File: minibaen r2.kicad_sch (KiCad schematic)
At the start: 134 parts, among them SW1 SW_Push, SW2 RotaryEncoder_Switch, U1 ATmega32U2-A, U2 PRTR5V0U2X, Y1 Crystal_GND24_Small

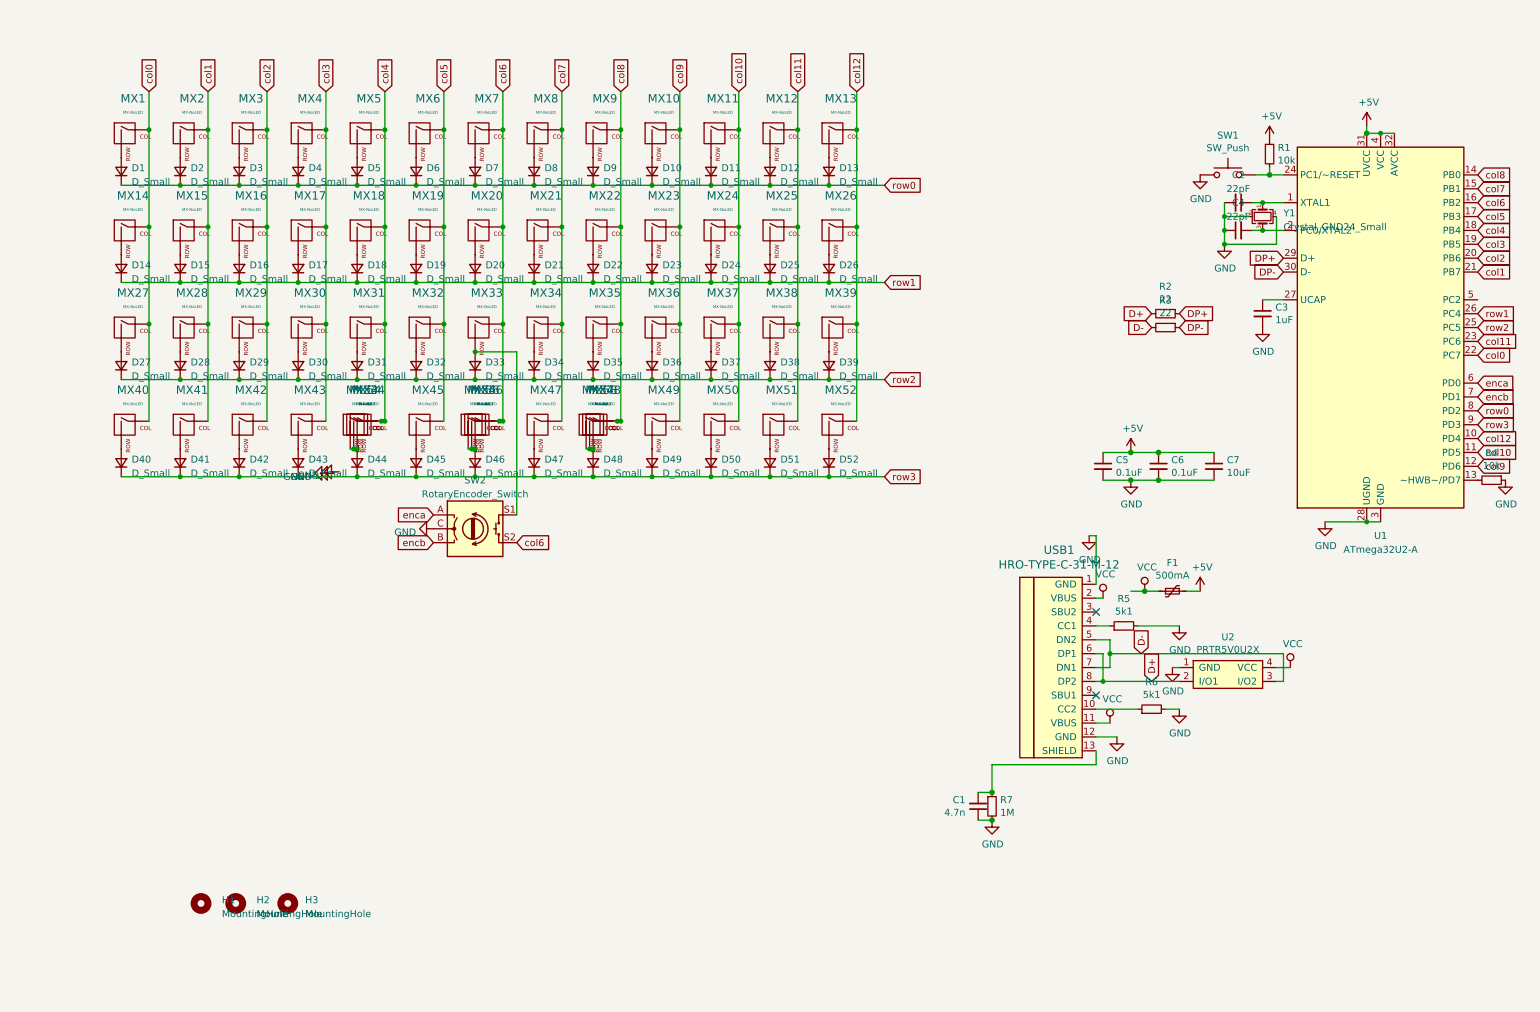
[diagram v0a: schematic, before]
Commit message: stagger
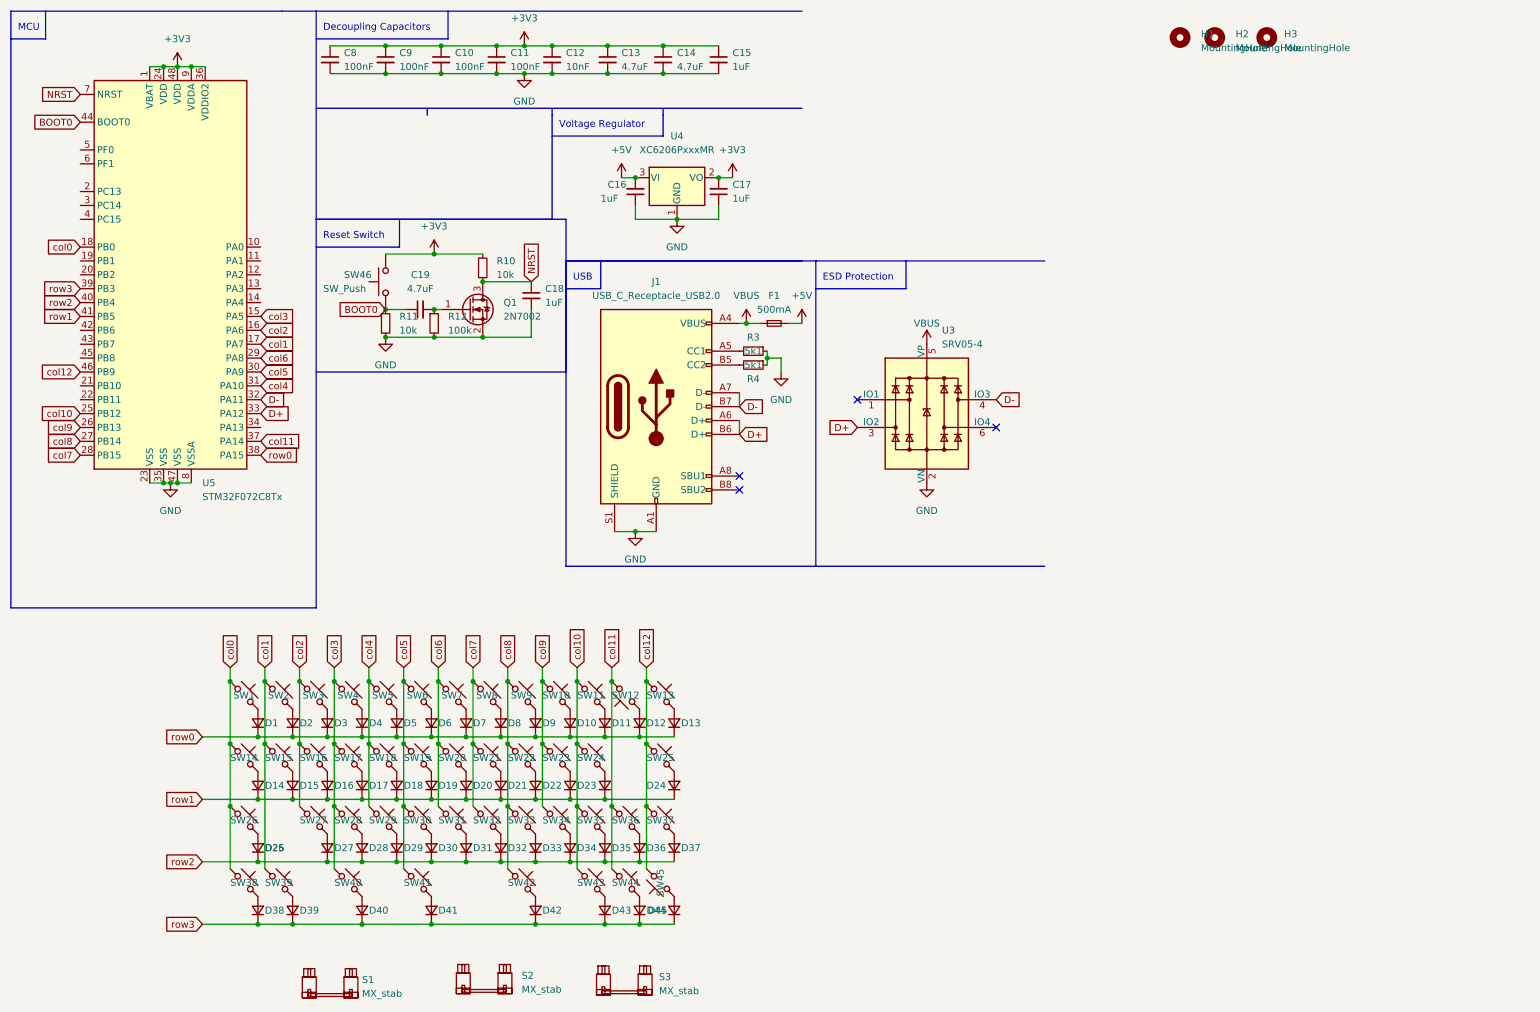
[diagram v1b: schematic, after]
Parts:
- removed C1: 4.7n, Capacitor_SMD:C_0603_1608Metric, symbol Device:C_Small
- removed C2, C4: 22pF, Capacitor_SMD:C_0603_1608Metric, symbol Device:C_Small
- removed C3: 1uF, Capacitor_SMD:C_0603_1608Metric, symbol Device:C_Small
- removed C5, C6: 0.1uF, Capacitor_SMD:C_0603_1608Metric, symbol Device:C_Small
- removed C7: 10uF, Capacitor_SMD:C_0603_1608Metric, symbol Device:C_Small
- removed D46, D47, D48, D49, D50, D51, D52: D_Small, Diode_SMD:D_SOD-123, symbol Device:D_Small
- removed F1: 500mA, Fuse:Fuse_1206_3216Metric, symbol Device:Polyfuse_Small
- removed MX1, MX10, MX11, MX12, MX13, MX14, MX15, MX16, MX17, MX18, MX19, MX2, MX20, MX21, MX22, MX23, MX24, MX25, MX26, MX27, MX28, MX29, MX3, MX30, MX31, MX32, MX33, MX34, MX35, MX36, MX37, MX38, MX39, MX4, MX40, MX41, MX42, MX43, MX44, MX45, MX46, MX47, MX48, MX49, MX5, MX50, MX51, MX52, MX6, MX7, MX8, MX9: MX-NoLED, MX_Only:MXOnly-1U-NoLED, symbol keybage:MX-NoLED
- removed MX53, MX57: MX-NoLED, MX_Only:MXOnly-2U-ReversedStabilizers-NoLED, symbol keybage:MX-NoLED
- removed MX54, MX56, MX58: MX-NoLED, MX_Only:MXOnly-3U-ReversedStabilizers-NoLED, symbol keybage:MX-NoLED
- removed MX55: MX-NoLED, MX_Only:MXOnly-7U-ReversedStabilizers-NoLED, symbol keybage:MX-NoLED
- removed R1: 10k, Resistor_SMD:R_0603_1608Metric, symbol Device:R_Small
- removed R2: 22, Resistor_SMD:R_0603_1608Metric, symbol Device:R_Small
- removed R5, R6: 5k1, Resistor_SMD:R_0603_1608Metric, symbol Device:R_Small
- removed R7: 1M, Resistor_SMD:R_0603_1608Metric, symbol Device:R_Small
- removed SW1: SW_Push, Connector_PinHeader_2.54mm:PinHeader_1x02_P2.54mm_Vertical, symbol Switch:SW_Push
- removed SW2: RotaryEncoder_Switch, keebio:RotaryEncoder_EC11-no-legs, symbol Device:RotaryEncoder_Switch
- removed U1: ATmega32U2-A, Package_QFP:TQFP-32_7x7mm_P0.8mm, symbol MCU_Microchip_ATmega:ATmega32U2-A
- removed U2: PRTR5V0U2X, Package_TO_SOT_SMD:SOT-143, symbol keebio:PRTR5V0U2X
- removed USB1: HRO-TYPE-C-31-M-12, Type-C:HRO-TYPE-C-31-M-12, symbol Type-C:HRO-TYPE-C-31-M-12
- removed Y1: Crystal_GND24_Small, Crystal:Crystal_SMD_3225-4Pin_3.2x2.5mm, symbol Device:Crystal_GND24_Small
- added C10, C11, C8, C9: 100nF, Capacitor_SMD:C_0402_1005Metric, symbol Device:C_Small
- added C12: 10nF, Capacitor_SMD:C_0402_1005Metric, symbol Device:C_Small
- added C13, C14, C19: 4.7uF, Capacitor_SMD:C_0402_1005Metric, symbol Device:C_Small
- added C15, C16, C17, C18: 1uF, Capacitor_SMD:C_0402_1005Metric, symbol Device:C_Small
- added F1: 500mA, Fuse:Fuse_0603_1608Metric, symbol Device:Fuse_Small
- added J1: USB_C_Receptacle_USB2.0, Connector_USB:USB_C_Receptacle_HRO_TYPE-C-31-M-12, symbol Connector:USB_C_Receptacle_USB2.0
- added Q1: 2N7002, Package_TO_SOT_SMD:SOT-23, symbol Transistor_FET:2N7002
- added R10, R11: 10k, Resistor_SMD:R_0402_1005Metric, symbol Device:R_Small
- added R12: 100k, Resistor_SMD:R_0402_1005Metric, symbol Device:R_Small
- added S1: MX_stab, marbastlib-mx:STAB_MX_2.75u, symbol marbastlib-mx:MX_stab
- added S2: MX_stab, marbastlib-mx:STAB_MX_3u, symbol marbastlib-mx:MX_stab
- added S3: MX_stab, marbastlib-mx:STAB_MX_2u, symbol marbastlib-mx:MX_stab
- added SW1, SW10, SW11, SW12, SW13, SW15, SW16, SW17, SW18, SW19, SW2, SW20, SW21, SW22, SW23, SW24, SW27, SW28, SW29, SW3, SW30, SW31, SW32, SW33, SW34, SW35, SW36, SW39, SW4, SW41, SW42, SW44, SW5, SW6, SW7, SW8, SW9: MX_SW_solder, marbastlib-mx:SW_MX_1u, symbol marbastlib-mx:MX_SW_solder
- added SW14, SW37, SW38, SW40, SW43, SW45: MX_SW_solder, marbastlib-mx:SW_MX_1.25u, symbol marbastlib-mx:MX_SW_solder
- added SW25, SW26: MX_SW_solder, marbastlib-mx:SW_MX_1.75u, symbol marbastlib-mx:MX_SW_solder
- added SW46: SW_Push, Button_Switch_SMD:SW_SPST_TL3342, symbol Switch:SW_Push
- added U3: SRV05-4, marbastlib-various:SOT-23-6-routable, symbol Power_Protection:SRV05-4
- added U4: XC6206PxxxMR, Package_TO_SOT_SMD:SOT-23, symbol Regulator_Linear:XC6206PxxxMR
- added U5: STM32F072C8Tx, Package_QFP:LQFP-48_7x7mm_P0.5mm, symbol MCU_ST_STM32F0:STM32F072C8Tx
- R3: value 22 -> 5k1; footprint Resistor_SMD:R_0603_1608Metric -> Resistor_SMD:R_0402_1005Metric
- R4: value 10k -> 5k1; footprint Resistor_SMD:R_0603_1608Metric -> Resistor_SMD:R_0402_1005Metric
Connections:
- net DP- is gone; now on net GND: R3.1
- net +5V: now also C16.2, F1.2, U4.3 (VI)
- net D+: now also J1.A6 (D+), J1.B6 (D+), U3.3 (IO2), U5.33 (PA12)
- net D-: now also J1.A7 (D-), J1.B7 (D-), U3.4 (IO3), U5.32 (PA11); no longer R3.2
- net GND: now also C10.2, C11.2, C12.2, C13.2, C14.2, C15.2, C16.1, C17.1, C18.2, C8.2, C9.2, J1.A1 (GND), J1.A12 (GND), J1.B1 (GND), J1.B12 (GND), J1.S1 (SHIELD), Q1.2 (S), R11.2, R12.2, U3.2 (VN), U4.1 (GND), U5.23 (VSS), U5.35 (VSS), U5.47 (VSS), U5.8 (VSSA)
- net col0: now also SW1.1, SW14.1, SW26.1, SW38.1, U5.18 (PB0)
- net col1: now also SW15.1, SW2.1, SW39.1, U5.17 (PA7)
- net col10: now also SW11.1, SW24.1, SW35.1, SW43.1, U5.25 (PB12)
- net col11: now also SW12.2, SW36.1, SW44.1, U5.37 (PA14)
- net col12: now also SW13.1, SW25.1, SW37.1, SW45.1, U5.46 (PB9)
- net col2: now also SW16.1, SW27.1, SW3.1, U5.16 (PA6)
- net col3: now also SW17.1, SW28.1, SW4.1, SW40.1, U5.15 (PA5)
- net col4: now also SW18.1, SW29.1, SW5.1, U5.31 (PA10)
- net col5: now also SW19.1, SW30.1, SW41.1, SW6.1, U5.30 (PA9)
- net col6: now also SW20.1, SW31.1, SW7.1, U5.29 (PA8)
- net col7: now also SW21.1, SW32.1, SW8.1, U5.28 (PB15)
- net col8: now also SW22.1, SW33.1, SW42.1, SW9.1, U5.27 (PB14)
- net col9: now also SW10.1, SW23.1, SW34.1, U5.26 (PB13)
- net row0: now also U5.38 (PA15)
- net row1: now also U5.41 (PB5); no longer D26.1 (K)
- net row2: now also D26.1 (K), U5.40 (PB4); no longer D38.1 (K), D39.1 (K)
- net row3: now also D38.1 (K), D39.1 (K), U5.39 (PB3)
- net at R4.2: now also J1.B5 (CC2)
- net at D43.2 (A): now also SW43.2
- net at D3.2 (A): now also SW3.2
- net at D39.2 (A): now also SW39.2
- net at D8.2 (A): now also SW8.2
- net at D25.2 (A): now also SW25.2
- net at D21.2 (A): now also SW21.2
- net at D2.2 (A): now also SW2.2
- net at D12.2 (A): now also SW12.1
- net at D33.2 (A): now also SW33.2
- net at D28.2 (A): now also SW28.2
- net at D19.2 (A): now also SW19.2
- net at D45.2 (A): now also SW45.2
- net at D38.2 (A): now also SW38.2
- net at D35.2 (A): now also SW35.2
- net at D22.2 (A): now also SW22.2
- net at D11.2 (A): now also SW11.2
- net at D1.2 (A): now also SW1.2
- net at D42.2 (A): now also SW42.2
- net at D13.2 (A): now also SW13.2
- net at D34.2 (A): now also SW34.2
- net at D7.2 (A): now also SW7.2
- net at D23.2 (A): now also SW23.2
- net at D41.2 (A): now also SW41.2
- net at D14.2 (A): now also SW14.2
- net at D40.2 (A): now also SW40.2
- net at D44.2 (A): now also SW44.2
- net at D24.2 (A): now also SW24.2
- net at D4.2 (A): now also SW4.2
- net at D15.2 (A): now also SW15.2
- net at D10.2 (A): now also SW10.2
- net at D9.2 (A): now also SW9.2
- net at D20.2 (A): now also SW20.2
- net at D16.2 (A): now also SW16.2
- net at D36.2 (A): now also SW36.2
- net at D6.2 (A): now also SW6.2
- net at D18.2 (A): now also SW18.2
- net at D31.2 (A): now also SW31.2
- net at D17.2 (A): now also SW17.2
- net at D30.2 (A): now also SW30.2
- net at D27.2 (A): now also SW27.2
- net at D5.2 (A): now also SW5.2
- net at D37.2 (A): now also SW37.2
- net at D32.2 (A): now also SW32.2
- net at D26.2 (A): now also SW26.2
- net at D29.2 (A): now also SW29.2
- new net: C19.2, Q1.1 (G), R12.1
- new net: J1.A5 (CC1), R3.2
- new net +3V3: C10.1, C11.1, C12.1, C13.1, C14.1, C15.1, C17.2, C8.1, C9.1, R10.1, SW46.2, U4.2 (VO), U5.1 (VBAT), U5.24 (VDD), U5.36 (VDDIO2), U5.48 (VDD), U5.9 (VDDA)
- new net BOOT0: C19.1, R11.1, SW46.1, U5.44 (BOOT0)
- new net NRST: C18.1, Q1.3 (D), R10.2, U5.7 (NRST)
- new net VBUS: F1.1, J1.A4 (VBUS), J1.A9 (VBUS), J1.B4 (VBUS), J1.B9 (VBUS), U3.5 (VP)
- no-connect marks 2 -> 4
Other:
- note added: "Decoupling Capacitors"
- note added: "ESD Protection"
- note added: "MCU"
- note added: "Reset Switch"
- note added: "USB"
- note added: "Voltage Regulator"
- moved on the sheet: H1, H2, H3
